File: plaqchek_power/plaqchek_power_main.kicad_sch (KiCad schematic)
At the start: 45 parts, among them U12 TPS54202DDC, U15 TPS62175DQC, U2 LM43601

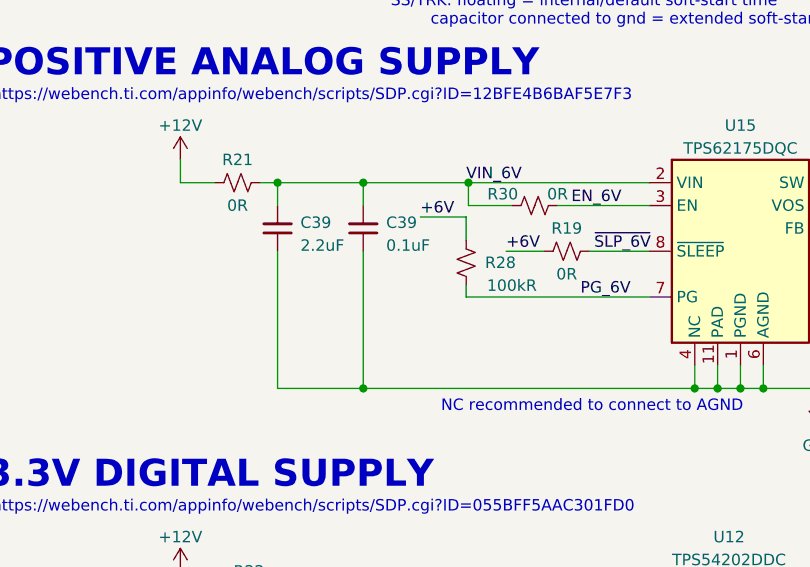
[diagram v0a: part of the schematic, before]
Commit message: finish all pcbs, generate gerber files
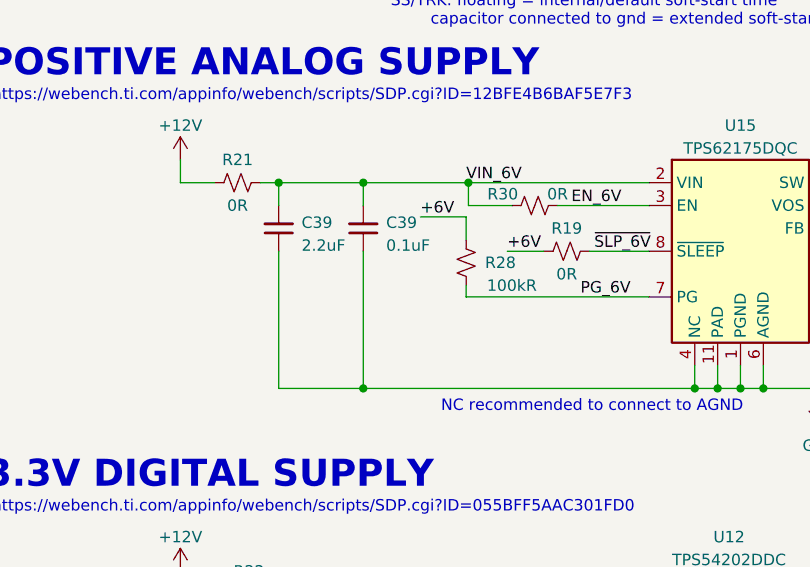
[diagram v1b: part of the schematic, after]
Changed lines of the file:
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@@
   (junction (at 151.13 167.64) (diameter 0) (color 0 0 0 0)
   )
-  (junction (at 52.705 107.95) (diameter 0) (color 0 0 0 0)
+  (junction (at 52.832 107.95) (diameter 0) (color 0 0 0 0)
   )
   (junction (at 205.74 83.82) (diameter 0) (color 0 0 0 0)
@@
     (stroke (width 0) (type default))
   )
-  (wire (pts (xy 52.705 107.95) (xy 52.705 110.49))
+  (wire (pts (xy 52.832 107.95) (xy 52.832 110.49))
     (stroke (width 0) (type default))
   )
@@
     (stroke (width 0) (type default))
   )
-  (wire (pts (xy 52.705 107.95) (xy 62.23 107.95))
+  (wire (pts (xy 52.832 107.95) (xy 62.23 107.95))
     (stroke (width 0) (type default))
   )
@@
     (stroke (width 0) (type default))
   )
-  (wire (pts (xy 52.705 107.95) (xy 50.8 107.95))
+  (wire (pts (xy 52.832 107.95) (xy 50.8 107.95))
     (stroke (width 0) (type default))
   )
@@
     (stroke (width 0) (type default))
   )
-  (wire (pts (xy 52.705 115.57) (xy 52.705 130.81))
+  (wire (pts (xy 52.832 115.57) (xy 52.832 130.81))
     (stroke (width 0) (type default))
   )
@@
     (stroke (width 0) (type default))
   )
-  (wire (pts (xy 52.705 130.81) (xy 62.23 130.81))
-    (stroke (width 0) (type default))
-  )
-  (wire (pts (xy 78.105 115.57) (xy 82.296 115.57))
+  (wire (pts (xy 52.832 130.81) (xy 62.23 130.81))
+    (stroke (width 0) (type default))
+  )
+  (wire (pts (xy 78.232 115.57) (xy 82.296 115.57))
     (stroke (width 0) (type default))
   )
@@
     (effects (font (size 1.27 1.27)) (justify left bottom))
   )
-  (label "+6V" (at 78.105 115.57 0) (fields_autoplaced)
+  (label "+6V" (at 78.232 115.57 0) (fields_autoplaced)
     (effects (font (size 1.27 1.27)) (justify left bottom))
   )
@@
     )
   )
-  (symbol (lib_id "Device:C_Small") (at 52.705 113.03 180) (unit 1)
-    (in_bom yes) (on_board yes) (dnp no) (fields_autoplaced)
-    (property "Reference" "C39" (at 55.245 112.3886 0)
+  (symbol (lib_id "Device:C_Small") (at 52.832 113.03 180) (unit 1)
+    (in_bom yes) (on_board yes) (dnp no) (fields_autoplaced)
+    (property "Reference" "C39" (at 55.372 112.3886 0)
       (effects (font (size 1.27 1.27)) (justify right))
     )
-    (property "Value" "2.2uF" (at 55.245 114.9286 0)
+    (property "Value" "2.2uF" (at 55.372 114.9286 0)
       (effects (font (size 1.27 1.27)) (justify right))
     )
-    (property "Footprint" "Capacitor_SMD:C_0603_1608Metric_Pad1.08x0.95mm_HandSolder" (at 52.705 113.03 0)
-      (effects (font (size 1.27 1.27)) hide)
-    )
-    (property "Datasheet" "~" (at 52.705 113.03 0)
-      (effects (font (size 1.27 1.27)) hide)
-    )
+    (property "Footprint" "Capacitor_SMD:C_0603_1608Metric_Pad1.08x0.95mm_HandSolder" (at 52.832 113.03 0)
+      (effects (font (size 1.27 1.27)) hide)
+    )
+    (property "Datasheet" "~" (at 52.832 113.03 0)
+      (effects (font (size 1.27 1.27)) hide)
+    )
